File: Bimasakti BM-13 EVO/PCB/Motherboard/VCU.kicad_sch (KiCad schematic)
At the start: 13 parts, among them J1 6437288-3, J10 Conn_01x02_Socket, J2 12V, J3 3V3_1, J4 3V3_2, J5 5V_1, J6 5V_2, J7 5V_3, J8 SIGNAL 1, J9 SIGNAL 2

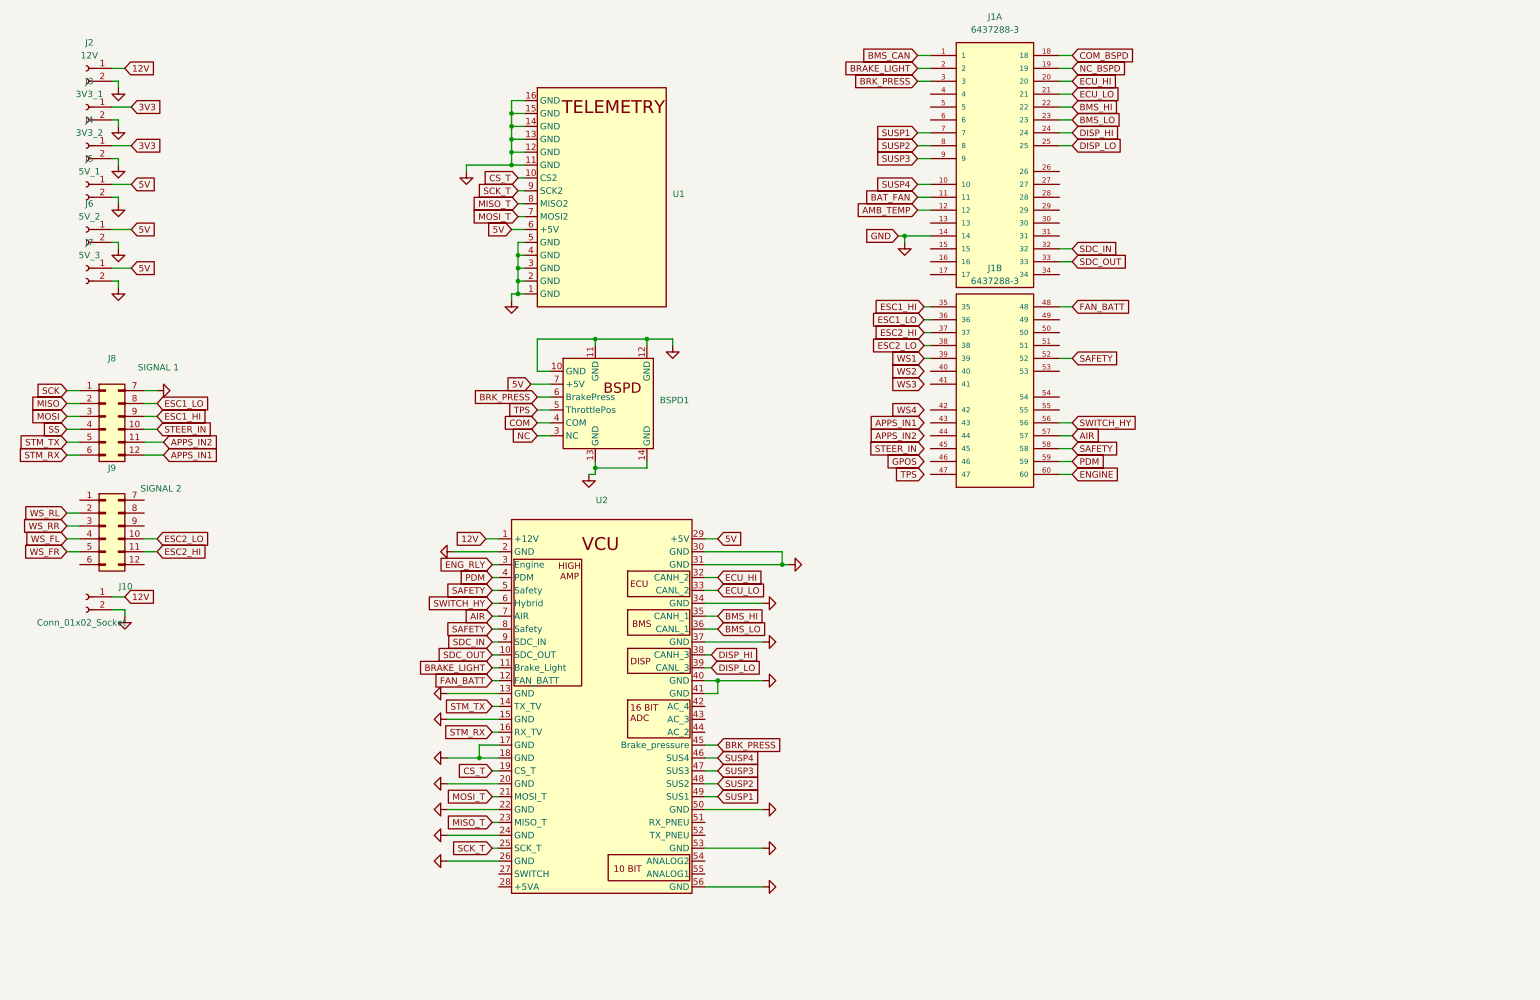
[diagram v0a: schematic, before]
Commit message: assembly VCU FINISH!!!
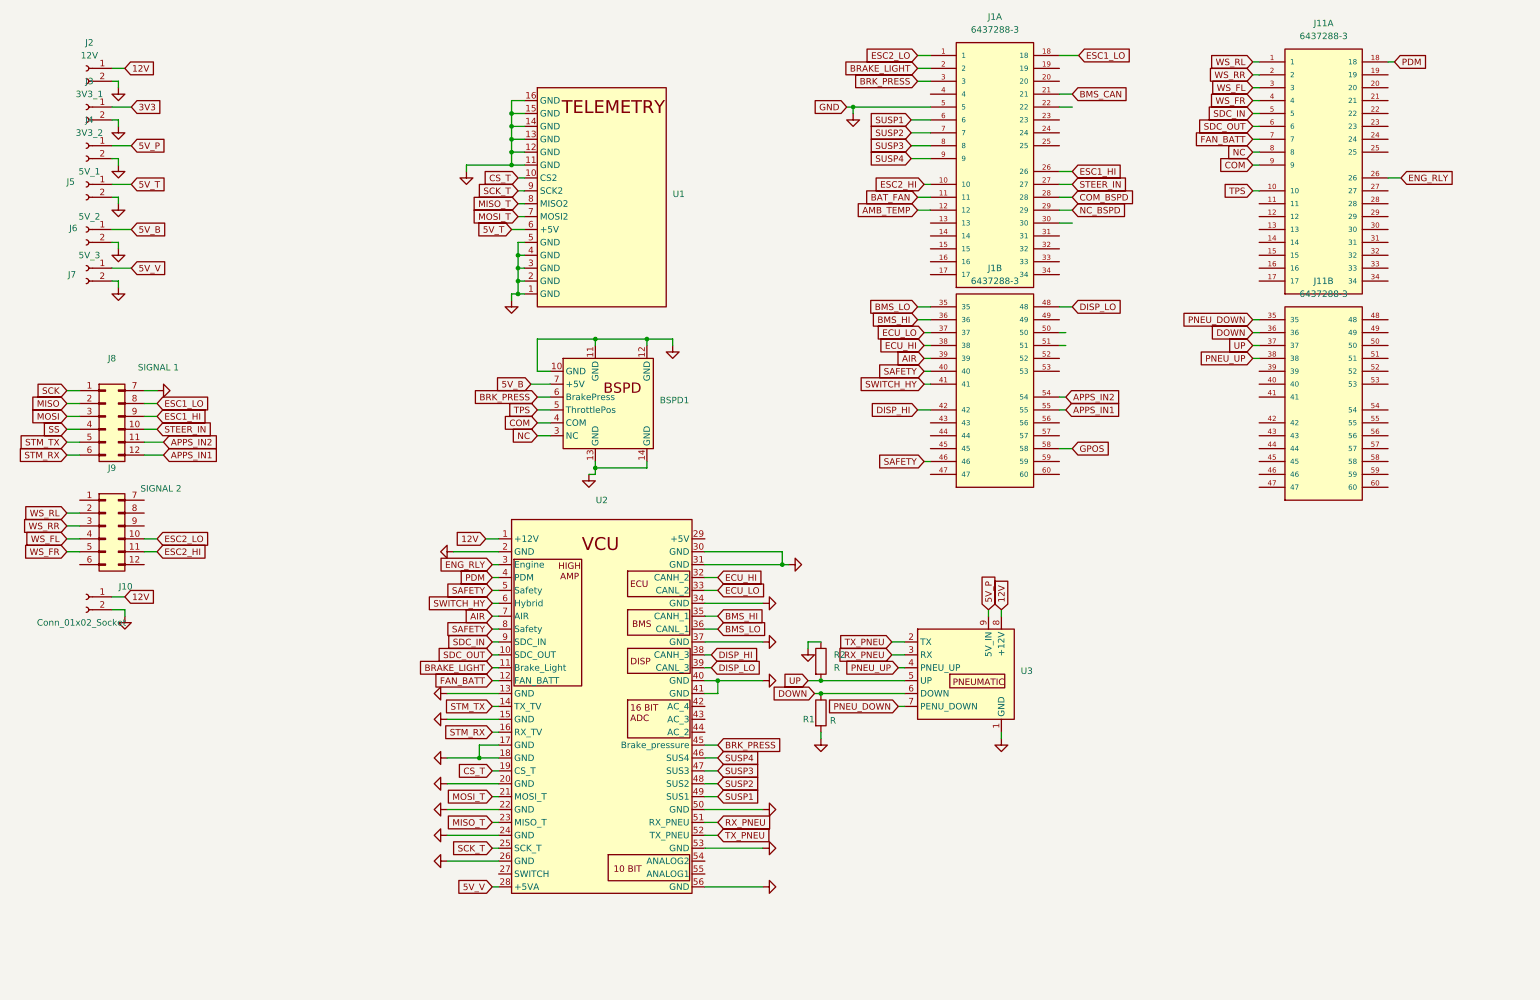
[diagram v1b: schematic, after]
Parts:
- added J11: 6437288-3, 0_VCU_CONNECTOR_TE_6437288-3:VCU_CONNECTOR_TE_6437288-3, symbol 0_VCU_connector_6437288-3:6437288-3
- added R1, R2: R, Resistor_SMD:R_0603_1608Metric_Pad0.98x0.95mm_HandSolder, symbol Device:R
- added U3: ~, 0_Footprint_PNEUMATIC:Fooprint Pneumatic, symbol 0_Pneumatic_Footprint:Pneumatic_Footprint
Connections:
- net WS1 is gone; now on net AIR: J1.39
- net 12V: now also U3.8 (+12V)
- net 3V3: no longer J4.1 (Pin_1)
- net AIR: no longer J1.57
- net APPS_IN1: now also J1.55
- net APPS_IN2: now also J1.54
- net BMS_CAN: now also J1.21; no longer J1.1
- net BMS_HI: now also J1.36; no longer J1.22
- net BMS_LO: now also J1.35; no longer J1.23
- net COM: now also J11.9
- net COM_BSPD: now also J1.28; no longer J1.18
- net DISP_HI: now also J1.42; no longer J1.24
- net DISP_LO: now also J1.48; no longer J1.25
- net ECU_HI: now also J1.38; no longer J1.20
- net ECU_LO: now also J1.37; no longer J1.21
- net ENG_RLY: now also J11.26
- net ESC1_HI: now also J1.26; no longer J1.35
- net ESC1_LO: now also J1.18; no longer J1.36
- net ESC2_HI: now also J1.10; no longer J1.37
- net ESC2_LO: now also J1.1; no longer J1.38
- net FAN_BATT: now also J11.7; no longer J1.48
- net GND: now also J1.5, R1.2, R2.1, U3.1 (GND); no longer J1.14
- net GPOS: now also J1.58
- net NC: now also J11.8
- net NC_BSPD: now also J1.29; no longer J1.19
- net PDM: now also J11.18; no longer J1.59
- net SAFETY: now also J1.40, J1.46; no longer J1.52, J1.58
- net SDC_IN: now also J11.5; no longer J1.32
- net SDC_OUT: now also J11.6; no longer J1.33
- net STEER_IN: now also J1.27
- net SUSP1: now also J1.6; no longer J1.7
- net SUSP2: now also J1.7; no longer J1.8
- net SUSP3: now also J1.8; no longer J1.9
- net SUSP4: now also J1.9; no longer J1.10
- net SWITCH_HY: now also J1.41; no longer J1.56
- net TPS: now also J11.10
- net WS_FL: now also J11.3
- net WS_FR: now also J11.4
- net WS_RL: now also J11.1
- net WS_RR: now also J11.2
- net 5V_V: now reaches U2.28 (+5VA)
- net 5V_V: now also J7.1 (Pin_1)
- net RX_PNEU: now reaches U2.51 (RX_PNEU)
- net RX_PNEU: now also U3.3 (RX)
- net TX_PNEU: now reaches U2.52 (TX_PNEU)
- net TX_PNEU: now also U3.2 (TX)
- removed net 5V: BSPD1.7 (+5V), J5.1 (Pin_1), J6.1 (Pin_1), J7.1 (Pin_1), U1.6 (+5V), U2.29 (+5V)
- net ENGINE: no longer names the net of J1.60
- new net 5V_B: BSPD1.7 (+5V), J6.1 (Pin_1)
- new net 5V_P: J4.1 (Pin_1), U3.9 (5V_IN)
- new net 5V_T: J5.1 (Pin_1), U1.6 (+5V)
- new net DOWN: J11.36, R1.1, U3.6 (DOWN)
- new net PNEU_DOWN: J11.35, U3.7 (PENU_DOWN)
- new net PNEU_UP: J11.38, U3.4 (PNEU_UP)
- new net UP: J11.37, R2.2, U3.5 (UP)

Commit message: update
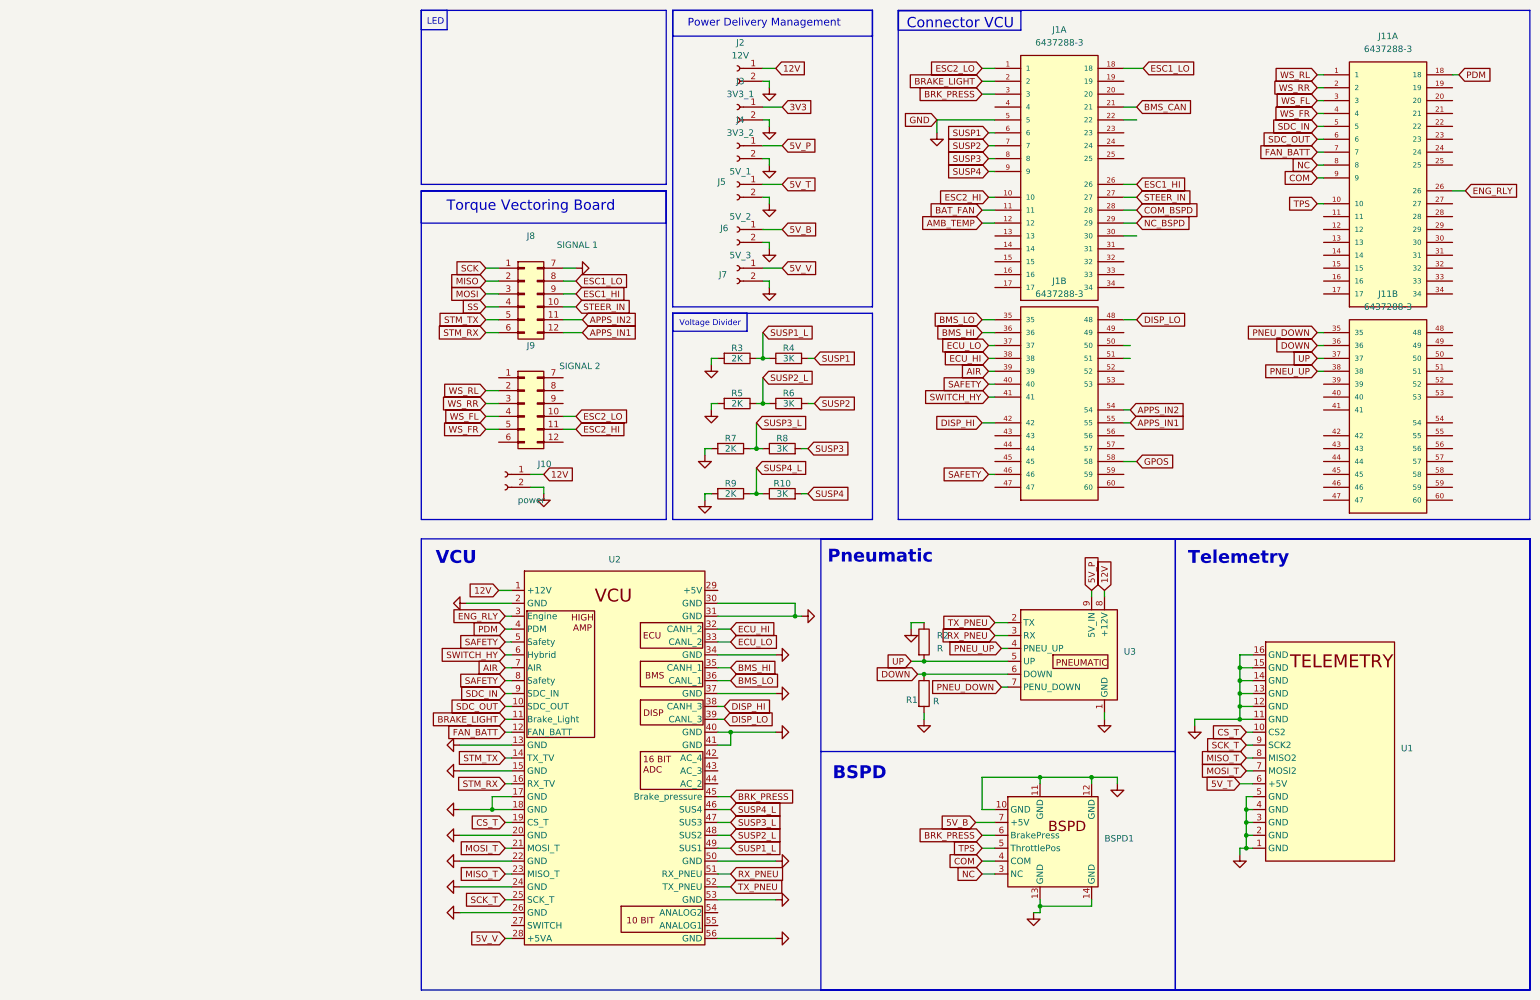
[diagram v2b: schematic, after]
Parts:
- added R10, R4, R6, R8: 3K, Resistor_SMD:R_0603_1608Metric_Pad0.98x0.95mm_HandSolder, symbol Device:R
- added R3, R5, R7, R9: 2K, Resistor_SMD:R_0603_1608Metric_Pad0.98x0.95mm_HandSolder, symbol Device:R
- J10: value Conn_01x02_Socket -> power
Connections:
- net GND: now also R3.2, R5.2, R7.2, R9.2
- net SUSP1: now also R4.2; no longer U2.49 (SUS1)
- net SUSP2: now also R6.2; no longer U2.48 (SUS2)
- net SUSP3: now also R8.2; no longer U2.47 (SUS3)
- net SUSP4: now also R10.2; no longer U2.46 (SUS4)
- new net SUSP1_L: R3.1, R4.1, U2.49 (SUS1)
- new net SUSP2_L: R5.1, R6.1, U2.48 (SUS2)
- new net SUSP3_L: R7.1, R8.1, U2.47 (SUS3)
- new net SUSP4_L: R10.1, R9.1, U2.46 (SUS4)
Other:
- note added: "BSPD"
- note added: "Connector VCU"
- note added: "LED"
- note added: "Pneumatic"
- note added: "Power Delivery Management"
- note added: "Telemetry"
- note added: "Torque Vectoring Board"
- note added: "VCU"
- note added: "Voltage Divider"
- moved on the sheet: BSPD1, J10, J11A, J11B, J1A, J1B, J2, J3, J4, J5, J6, J7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

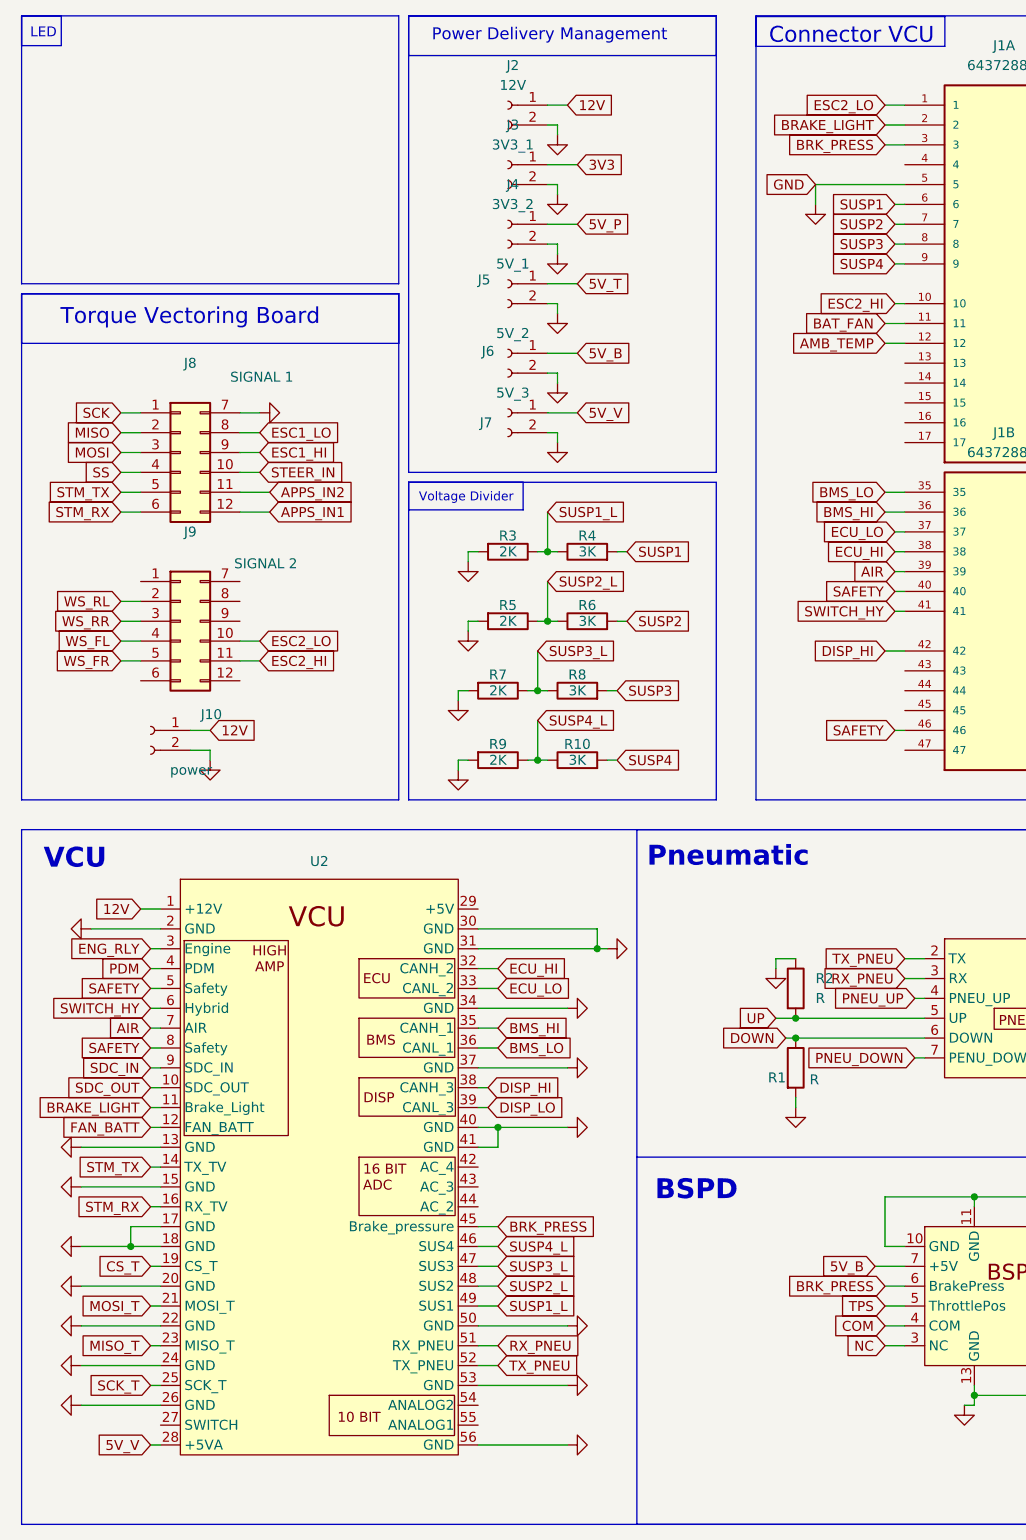
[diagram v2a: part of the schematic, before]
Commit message: detailing
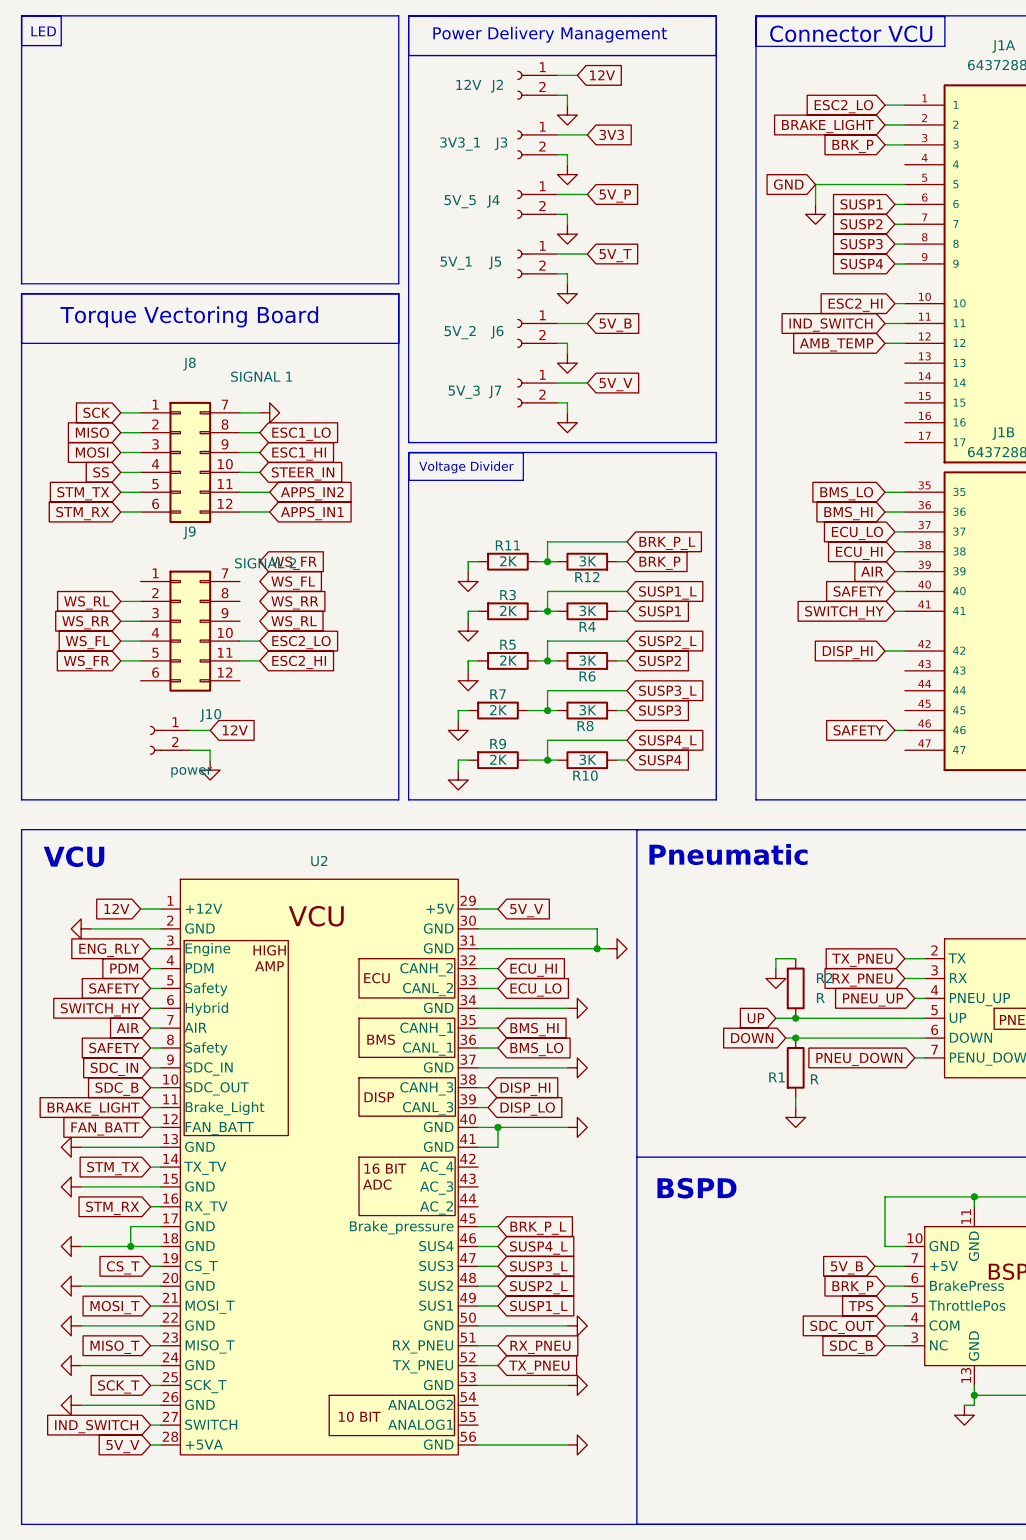
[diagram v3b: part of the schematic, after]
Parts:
- added R11: 2K, Resistor_SMD:R_0603_1608Metric_Pad0.98x0.95mm_HandSolder, symbol Device:R
- added R12: 3K, Resistor_SMD:R_0603_1608Metric_Pad0.98x0.95mm_HandSolder, symbol Device:R
- J4: value 3V3_2 -> 5V_5
- R3: footprint Resistor_SMD:R_0603_1608Metric_Pad0.98x0.95mm_HandSolder -> BRK_Press
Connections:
- net BAT_FAN is gone; now on net IND_SWITCH: J1.11
- net 5V_V: now also U2.29 (+5V)
- net COM: no longer BSPD1.4 (COM)
- net GND: now also R11.2
- net NC: no longer BSPD1.3 (NC)
- net SDC_OUT: now also BSPD1.4 (COM); no longer U2.10 (SDC_OUT)
- net IND_SWITCH: now reaches U2.27 (SWITCH)
- net BRK_PRESS renamed BRK_P
- net BRK_P: now also R12.2; no longer U2.45 (Brake_pressure)
- new net BRK_P_L: R11.1, R12.1, U2.45 (Brake_pressure)
- new net SDC_B: BSPD1.3 (NC), U2.10 (SDC_OUT)
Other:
- moved on the sheet: J2, J3, J4, J5, J6, J7, R10, R3, R4, R5, R6, R7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
